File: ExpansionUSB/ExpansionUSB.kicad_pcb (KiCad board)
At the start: 2 copper layers, 54.5 x 64 mm, 12 parts, among them J1 USB_A, J2 USB_A_PTH_MALE, J3 USB_A, J4 USB_A_PTH_MALE, U1 ACS712xLCTR-05B, U2 ACS712xLCTR-05B, U3 NodeMCU_1.0_(ESP-12E), U4 CD4051B

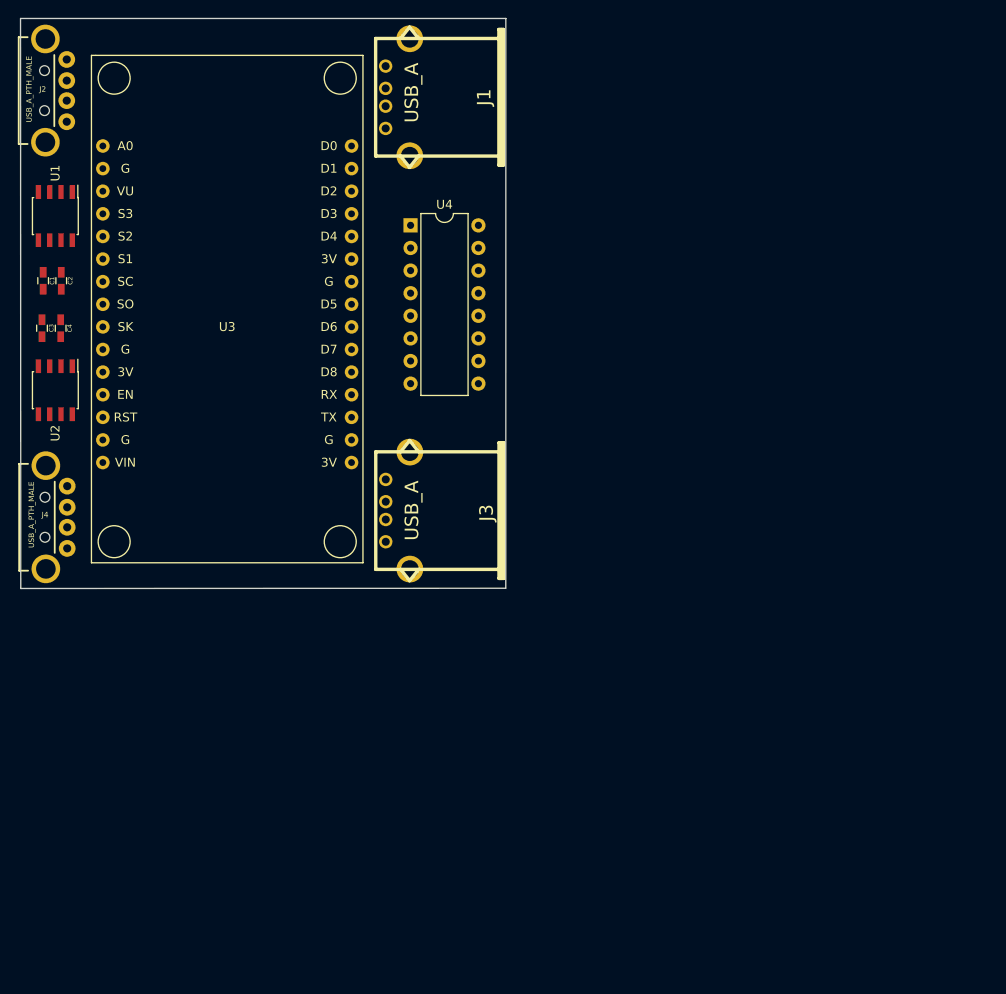
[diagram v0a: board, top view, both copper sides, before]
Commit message: final usb expansion
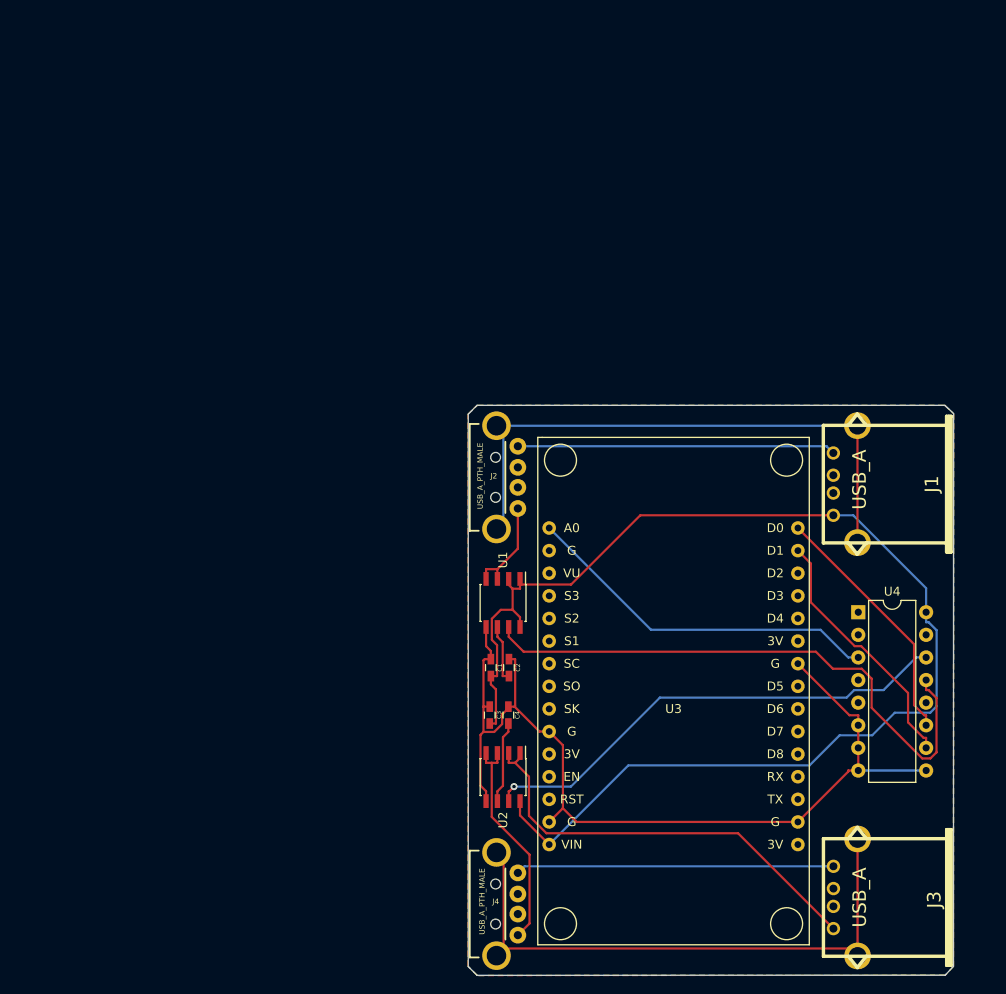
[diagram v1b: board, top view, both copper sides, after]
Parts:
- moved J2 66.7 mm to (117.0, 74.4)
- moved J4 66.7 mm to (117.0, 122.3)
- moved U1 66.5 mm to (117.7, 88.5)
- moved U2 66.5 mm to (117.7, 108.1)
- moved J1 66.5 mm to (160.8, 75.2)
- moved C3 66.5 mm to (116.2, 101.1)
- moved C2 66.5 mm to (118.4, 95.8)
- moved U4 66.5 mm to (157.6, 89.6)
- moved C1 66.5 mm to (116.3, 95.8)
- moved J3 66.5 mm to (160.8, 121.6)
- moved C4 66.5 mm to (118.3, 101.1)
- moved U3 66.0 mm to (136.9, 100.4)
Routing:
- net +5V: track 0.00 -> 146.6 mm
- net GND: track 0.00 -> 108.9 mm
- net Net-(U1-Pad7): track 0.00 -> 65.8 mm
- net Net-(J1-Pad5): track 0.00 -> 65.6 mm
- net Net-(J3-Pad5): track 0.00 -> 65.2 mm
- net Net-(U2-Pad7): track 0.00 -> 54.2 mm, vias 0 -> 1
- net Net-(J3-Pad1): track 0.00 -> 49.2 mm
- net Net-(U3-Pad1): track 0.00 -> 40.7 mm
- net Net-(J3-Pad4): track 0.00 -> 35.8 mm
- net Net-(J1-Pad4): track 0.00 -> 35.8 mm
- net Net-(U3-Pad29): track 0.00 -> 28.7 mm
- net Net-(U3-Pad30): track 0.00 -> 28.3 mm
- net Net-(J4-PadVBUS): track 0.00 -> 25.1 mm
- net Net-(J2-PadVBUS): track 0.00 -> 11.2 mm
- net Net-(C4-Pad2): track 0.00 -> 9.22 mm
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- added copper zone on B.Cu, net GND
- added copper zone on F.Cu, net GND
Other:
- outline, holes or cut-outs redrawn

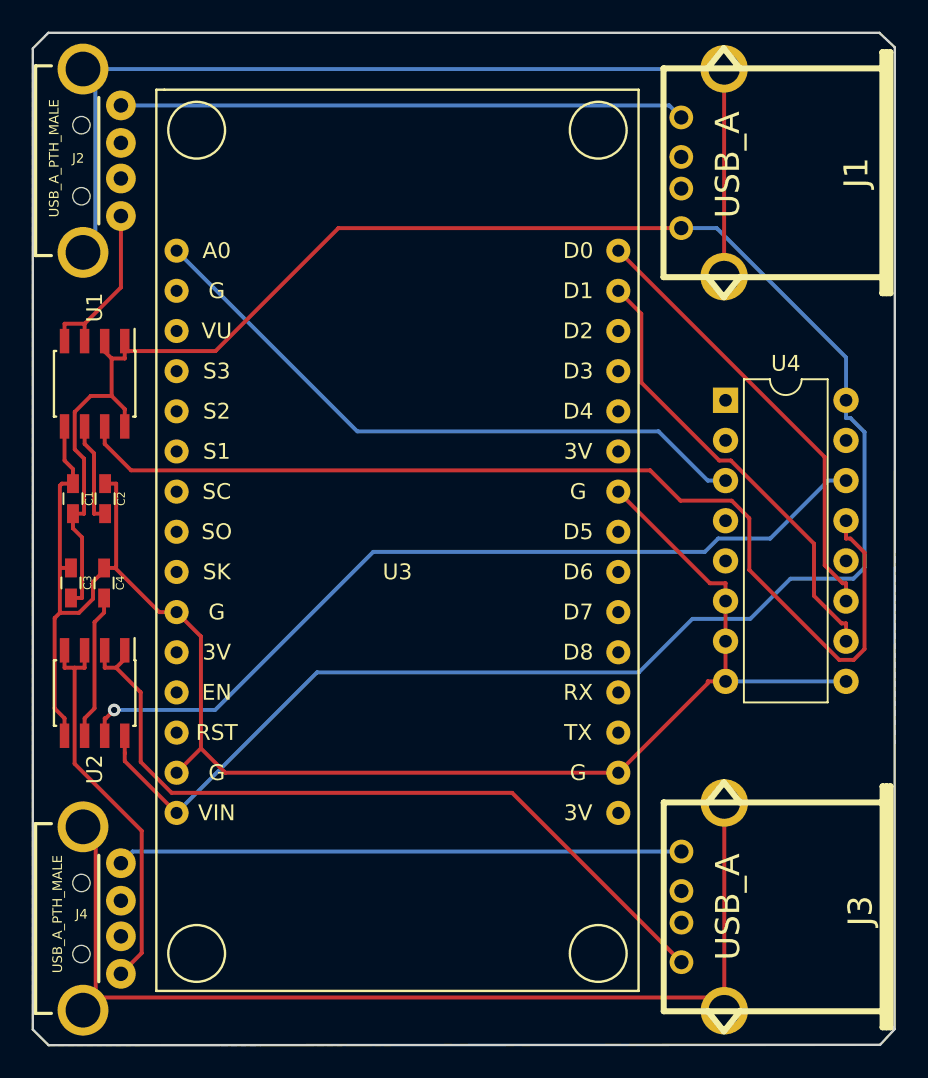
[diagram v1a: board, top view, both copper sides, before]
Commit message: Actualización tarjetas
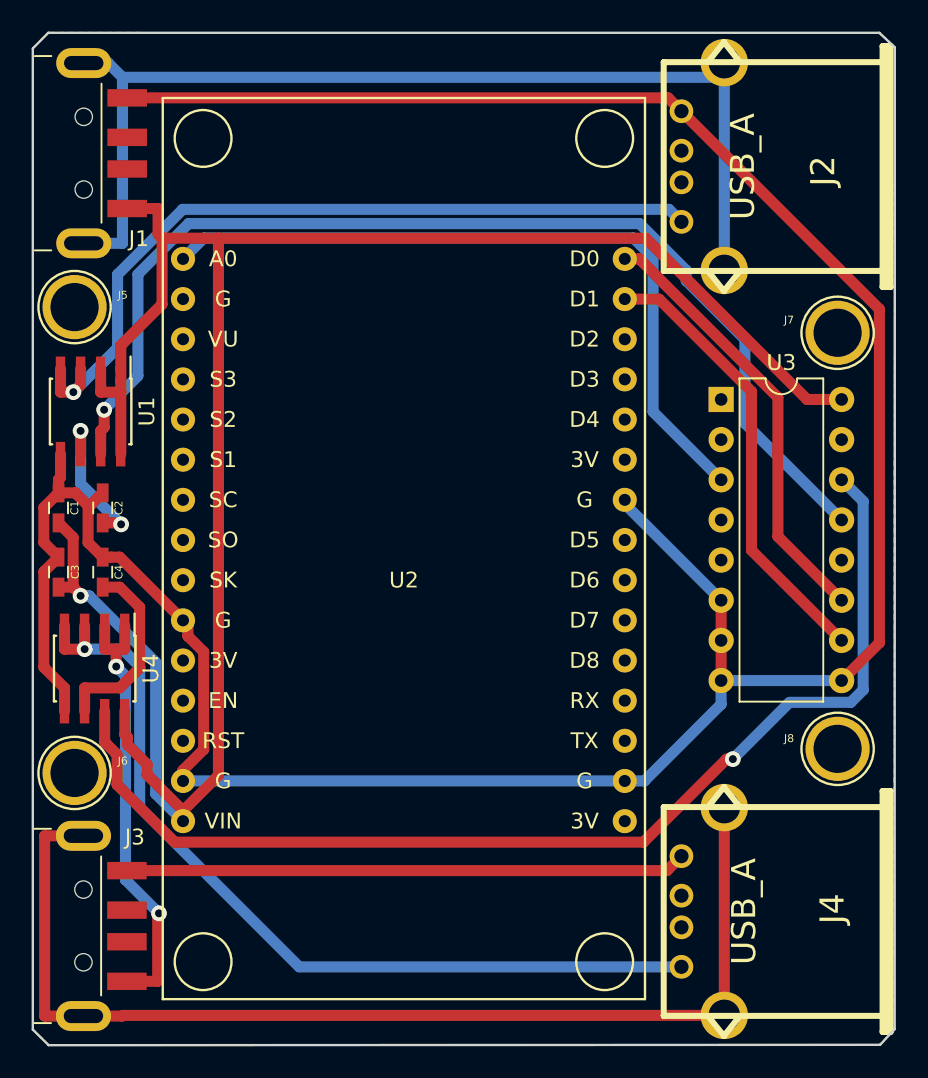
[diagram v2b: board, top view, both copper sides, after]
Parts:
- added J5: H1, Socket_Arduino_Uno:Arduino_1pin, F.Cu at (116.4, 83.7)
- added J6: H2, Socket_Arduino_Uno:Arduino_1pin, F.Cu at (116.4, 113.1)
- added J7: H3, Socket_Arduino_Uno:Arduino_1pin, F.Cu at (164.7, 85.3)
- added J8: H4, Socket_Arduino_Uno:Arduino_1pin, F.Cu at (164.7, 111.6)
- J1, J3: footprint w_conn_pc:conn_usb_A -> Connector_USB:USB_A_CNCTech_1001-011-01101_Horizontal
- J2, J4: value USB_A_PTH_MALE -> USB_A; footprint Connectors:USB-A-H -> w_conn_pc:conn_usb_A
- U2: value ACS712xLCTR-05B -> NodeMCU_1.0_(ESP-12E); footprint Package_SO:SOIC-8_3.9x4.9mm_P1.27mm -> ESP8266:NodeMCU-LoLinV3
- U3: value NodeMCU_1.0_(ESP-12E) -> CD4051B; footprint ESP8266:NodeMCU-LoLinV3 -> Housings_DIP:DIP-16_W7.62mm
- U4: value CD4051B -> ACS712xLCTR-05B; footprint Housings_DIP:DIP-16_W7.62mm -> Package_SO:SOIC-8_3.9x4.9mm_P1.27mm
- moved J3 50.7 mm to (110.1, 122.8), turned to 180 degrees
- moved J1 50.7 mm to (110.1, 73.9), turned to 180 degrees
- moved J4 43.8 mm to (160.8, 121.9), turned to 90 degrees
- moved J2 43.8 mm to (160.8, 74.8), turned to 90 degrees
- moved U4 43.4 mm to (117.7, 106.5), turned to 270 degrees
- moved U3 23.2 mm to (157.3, 89.5)
- moved U2 20.8 mm to (137.3, 100.9), turned to 0 degrees
- moved U1 1.77 mm to (117.5, 90.3)
- moved C1 1.08 mm to (115.4, 96.4)
- moved C3 1.04 mm to (115.4, 100.4)
- moved C4 0.69 mm to (118.2, 100.4)
- moved C2 0.60 mm to (118.2, 96.4)
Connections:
- J1 pad 4: Net-(J1-Pad4) -> GND
- U1 pad 3: Net-(J2-PadVBUS) -> Net-(J2-Pad1)
- U1 pad 4: Net-(J2-PadVBUS) -> Net-(J2-Pad1)
- U2 pad 1: Net-(J3-Pad1) -> Net-(U2-Pad1)
- U2 pad 2: Net-(J3-Pad1) -> (no net)
- U2 pad 3: Net-(J4-PadVBUS) -> (no net)
- U2 pad 4: Net-(J4-PadVBUS) -> (no net)
- U2 pad 5: GND -> (no net)
- U2 pad 6: Net-(C4-Pad2) -> (no net)
- U2 pad 7: Net-(U2-Pad7) -> (no net)
- U2 pad 8: +5V -> (no net)
- U3 pad 1: Net-(U3-Pad1) -> (no net)
- U3 pad 10: GND -> Net-(U2-Pad29)
- U3 pad 11: (no net) -> Net-(U2-Pad30)
- U3 pad 13: (no net) -> Net-(U1-Pad7)
- U3 pad 14: GND -> Net-(U3-Pad14)
- U3 pad 15: +5V -> (no net)
- U3 pad 16: (no net) -> +5V
- U3 pad 3: (no net) -> Net-(U2-Pad1)
- U3 pad 6: (no net) -> GND
- U3 pad 7: (no net) -> GND
- U3 pad 8: (no net) -> GND
- U3 pad 9: (no net) -> GND
- U4 pad 1: (no net) -> Net-(J3-Pad1)
- U4 pad 2: (no net) -> Net-(J3-Pad1)
- U4 pad 3: Net-(U3-Pad1) -> Net-(J4-Pad1)
- U4 pad 4: (no net) -> Net-(J4-Pad1)
- U4 pad 5: (no net) -> GND
- U4 pad 6: GND -> Net-(C4-Pad2)
- U4 pad 7: GND -> Net-(U3-Pad14)
- U4 pad 8: GND -> +5V
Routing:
- net Net-(U3-Pad14): track 0.00 -> 71.5 mm, vias 0 -> 1
- net GND: track 108.9 -> 179.8 mm
- net Net-(J4-Pad1): track 0.00 -> 55.5 mm, vias 0 -> 1
- net Net-(U2-Pad7): track 54.2 -> 0.00 mm, vias 1 -> 0
- net Net-(J2-Pad1): track 0.00 -> 50.3 mm, vias 0 -> 1
- net Net-(U2-Pad1): track 0.00 -> 46.6 mm
- net Net-(U3-Pad1): track 40.7 -> 0.00 mm
- net Net-(J1-Pad4): track 35.8 -> 0.00 mm
- net Net-(U3-Pad29): track 28.7 -> 0.00 mm
- net Net-(U2-Pad29): track 0.00 -> 28.5 mm
- net Net-(U3-Pad30): track 28.3 -> 0.00 mm
- net Net-(U2-Pad30): track 0.00 -> 27.8 mm
- net Net-(J4-PadVBUS): track 25.1 -> 0.00 mm
- net Net-(J3-Pad1): track 49.2 -> 28.3 mm, vias 0 -> 2
- net Net-(J2-PadVBUS): track 11.2 -> 0.00 mm
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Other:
- net class Default: trace_width 0.25 -> 0.7; via_dia 0.8 -> 1; via_drill 0.4 -> 0.6

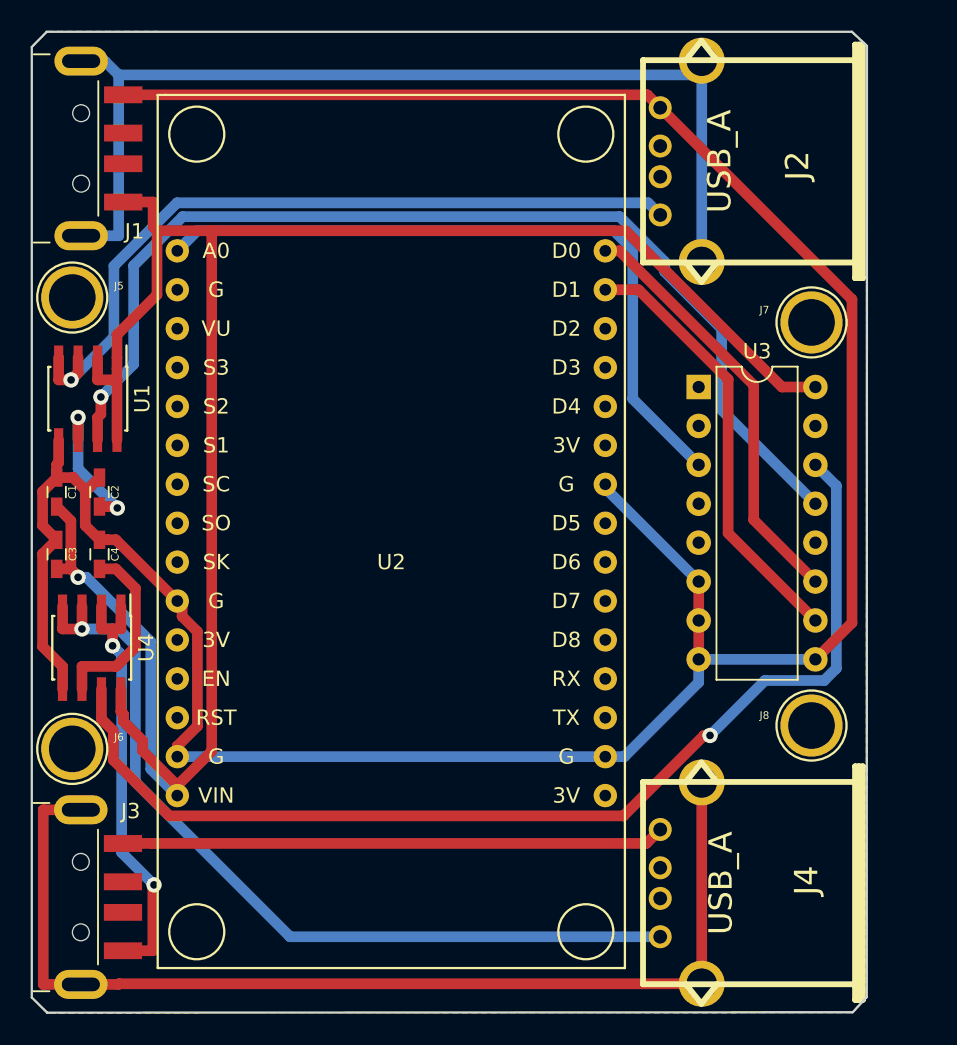
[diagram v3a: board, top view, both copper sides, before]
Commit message: Update expansion
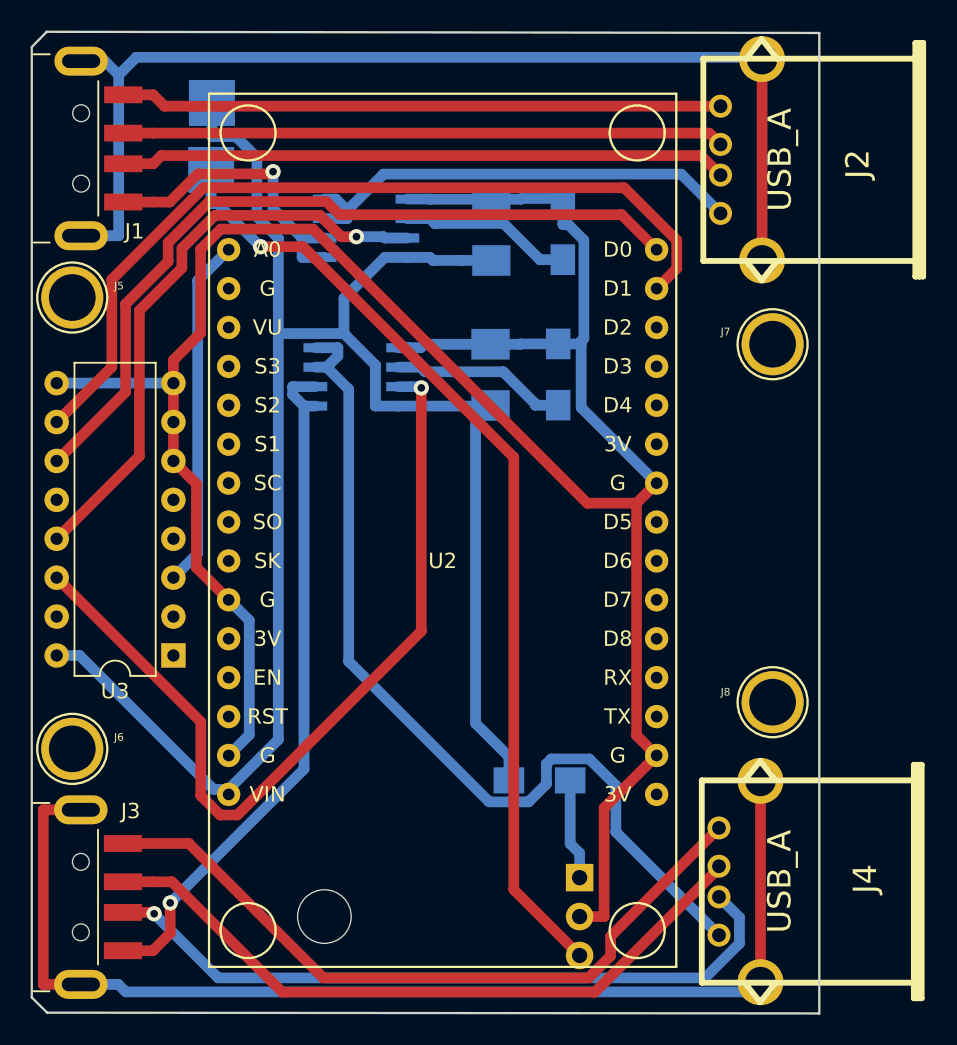
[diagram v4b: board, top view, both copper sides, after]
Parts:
- added GND1: HEART, Measurement_Points:Measurement_Point_Square-SMD-Pad_Big, B.Cu at (125.5, 75.3)
- added Q1: IRF640N, TO_SOT_Packages_THT:TO-220_Horizontal, B.Cu at (149.6, 121.5)
- added R1: 10K, Resistors_SMD:R_1206_HandSoldering, B.Cu at (146.9, 115.2)
- added VCC1: +5V, Measurement_Points:Measurement_Point_Square-SMD-Pad_Big, B.Cu at (125.6, 71.0)
- C1, C3: footprint Capacitors_SMD:C_0603_HandSoldering -> Capacitors_SMD:C_1210_HandSoldering; moved to B.Cu
- C2, C4: footprint Capacitors_SMD:C_0603_HandSoldering -> Capacitors_SMD:C_1206_HandSoldering; moved to B.Cu
- U1, U4: moved to B.Cu
- moved U3 38.5 mm to (123.0, 107.0), turned to 180 degrees
- moved C2 34.8 mm to (148.5, 79.2)
- moved C1 33.1 mm to (143.8, 79.2)
- moved C4 32.2 mm to (148.2, 88.7)
- moved C3 30.6 mm to (143.7, 88.7)
- moved U4 24.7 mm to (135.0, 88.8), turned to 0 degrees
- moved U1 21.3 mm to (135.6, 79.1), turned to 0 degrees
- moved J2 3.94 mm to (164.7, 74.7)
- moved J4 3.84 mm to (164.6, 121.8)
- moved U2 3.35 mm to (140.6, 100.9)
- moved J8 2.96 mm to (162.2, 110.1)
- moved J7 2.91 mm to (162.2, 86.7)
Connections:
- J1 pad 1: +5V -> Net-(J1-Pad1)
- J1 pad 2: (no net) -> Net-(J1-Pad2)
- J1 pad 3: (no net) -> Net-(J1-Pad3)
- J1 pad 4: GND -> Net-(J1-Pad4)
- J2 pad 2: (no net) -> Net-(J1-Pad2)
- J2 pad 3: (no net) -> Net-(J1-Pad3)
- J2 pad 4: GND -> Net-(J1-Pad4)
- J3 pad 2: (no net) -> Net-(J3-Pad2)
- J3 pad 3: (no net) -> Net-(J3-Pad3)
- J4 pad 2: (no net) -> Net-(J3-Pad2)
- J4 pad 3: (no net) -> Net-(J3-Pad3)
- U1 pad 1: +5V -> Net-(J1-Pad1)
- U1 pad 2: +5V -> Net-(J1-Pad1)
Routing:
- net Net-(GND1-Pad1): track 0.00 -> 63.1 mm, vias 0 -> 1
- net Net-(J3-Pad2): track 0.00 -> 46.5 mm, vias 0 -> 1
- net Net-(J3-Pad3): track 0.00 -> 45.4 mm
- net Net-(J1-Pad2): track 0.00 -> 39.7 mm
- net Net-(J1-Pad4): track 0.00 -> 39.3 mm
- net Net-(J1-Pad3): track 0.00 -> 39.3 mm
- net Net-(U1-Pad7): track 69.4 -> 38.6 mm
- net Net-(U2-Pad29): track 28.5 -> 55.3 mm
- net Net-(U2-Pad30): track 27.8 -> 51.6 mm
- net Net-(U2-Pad1): track 46.6 -> 22.9 mm
- net GND: track 179.8 -> 156.6 mm
- net Net-(J2-Pad1): track 50.3 -> 30.2 mm, vias 1 -> 0
- net Net-(J1-Pad1): track 0.00 -> 19.9 mm, vias 0 -> 1
- net +5V: track 137.6 -> 119.9 mm, vias 1 -> 0
- net Net-(J3-Pad1): track 28.3 -> 45.4 mm, vias 2 -> 1
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- removed copper zone on B.Cu, net GND
- removed copper zone on F.Cu, net GND
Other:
- board size 54.5 x 64 mm -> 51.4 x 64.1 mm
